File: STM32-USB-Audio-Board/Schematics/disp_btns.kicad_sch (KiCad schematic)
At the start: 8 parts, among them J8 Conn_01x08, J9 Conn_01x05

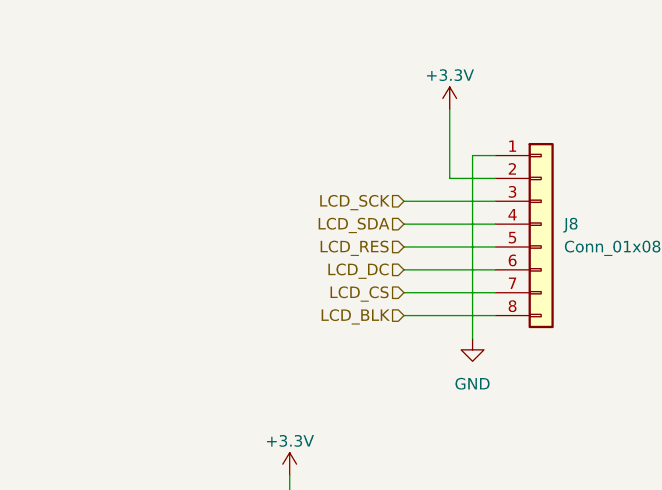
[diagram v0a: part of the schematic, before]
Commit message: Cleanup
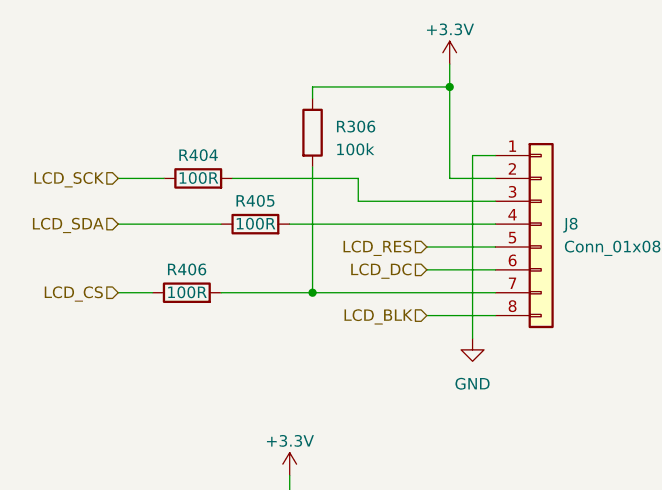
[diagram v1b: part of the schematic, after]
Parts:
- added R306: 100k, Resistor_SMD:R_0402_1005Metric, symbol Device:R
- added R404, R405, R406: 100R, Resistor_SMD:R_0402_1005Metric, symbol Device:R
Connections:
- net +3.3V: now also R306.1
- net LCD_CS: now also R406.1; no longer J8.7 (Pin_7)
- net LCD_SCK: now also R404.1; no longer J8.3 (Pin_3)
- net LCD_SDA: now also R405.1; no longer J8.4 (Pin_4)
- new net: J8.7 (Pin_7), R306.2, R406.2
- new net: J8.3 (Pin_3), R404.2
- new net: J8.4 (Pin_4), R405.2
